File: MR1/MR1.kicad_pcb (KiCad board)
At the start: 2 copper layers, 94 x 71.1 mm, 16 parts, among them J1 Conn_01x04_Male, J2 Conn_01x04_Male, J3 Conn_01x04_Male, J4 Conn_01x04_Male, J5 Conn_01x02_Male, J6 Conn_01x04_Male, J7 Conn_01x04_Male, J8 Conn_01x04_Male, Q1 2SC1815, U5 LPC1768, U6 MPU6050, U7 R3008SB, U8 MCP2561-E-P

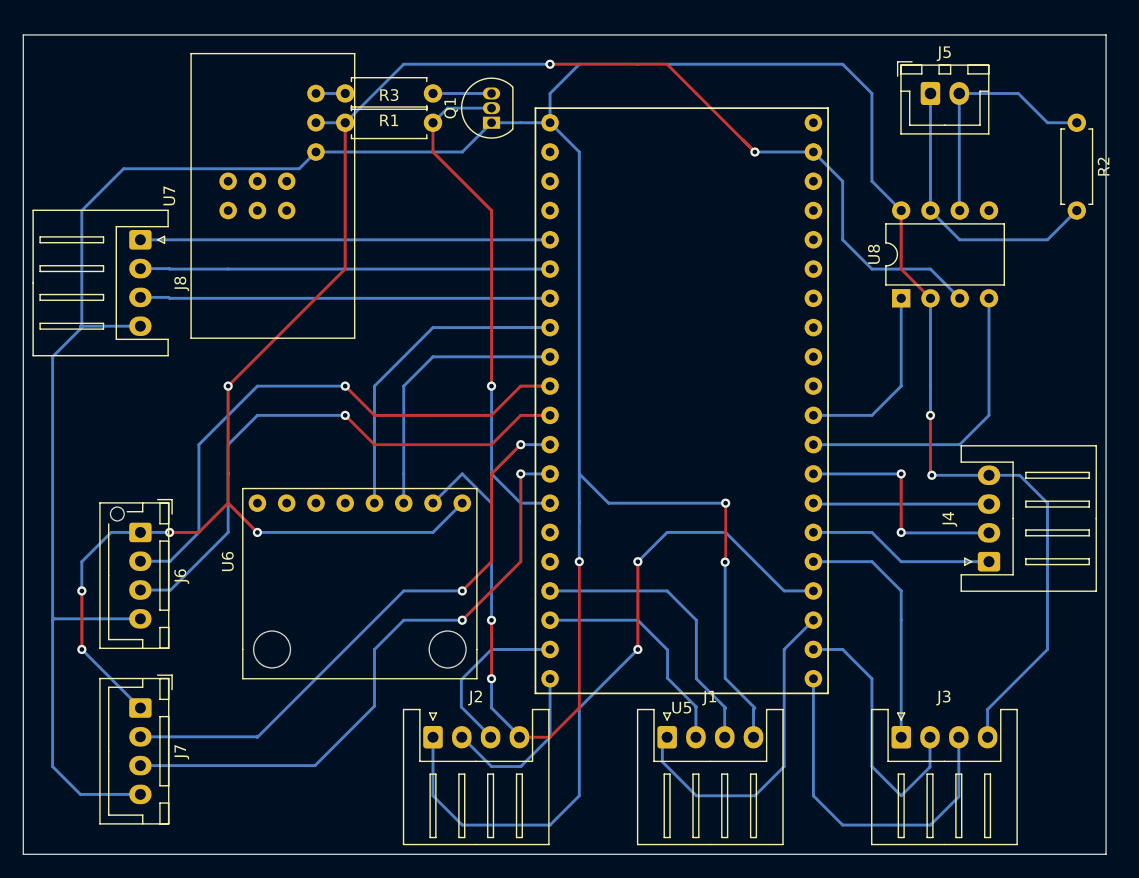
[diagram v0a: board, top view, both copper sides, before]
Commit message: fix: MR1
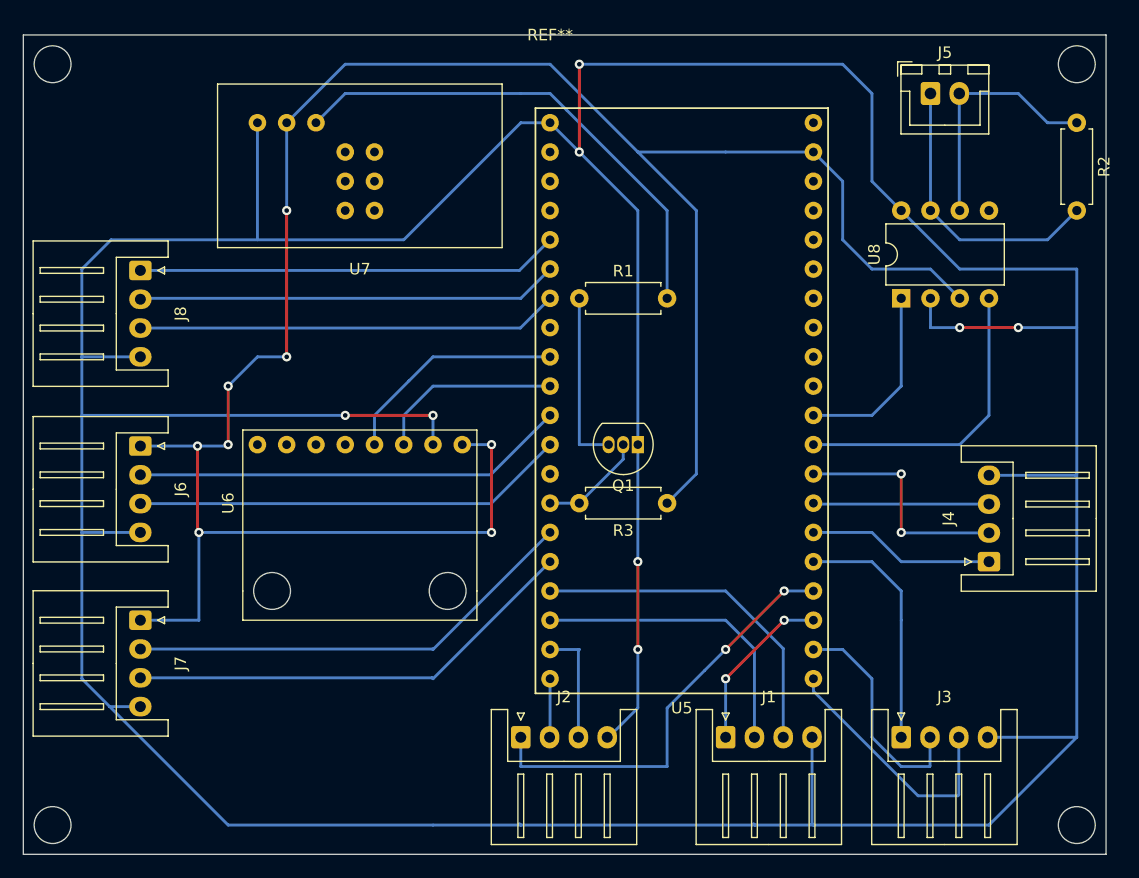
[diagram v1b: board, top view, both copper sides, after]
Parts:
- added REF**: universal_B, MyFootprint:universal_B, F.Cu at (142.2, 99.1)
- J6: footprint Connector_JST:JST_XH_B4B-XH-AM_1x04_P2.50mm_Vertical -> Connector_JST:JST_XH_S4B-XH-A_1x04_P2.50mm_Horizontal
- J7: footprint Connector_JST:JST_XH_B4B-XH-A_1x04_P2.50mm_Vertical -> Connector_JST:JST_XH_S4B-XH-A_1x04_P2.50mm_Horizontal
- moved R3 43.3 mm to (152.4, 104.1), turned to 180 degrees
- moved Q1 30.7 mm to (149.9, 99.1), turned to 180 degrees
- moved R1 21.8 mm to (144.8, 86.4), turned to 0 degrees
- moved J7 7.62 mm to (106.7, 114.3)
- moved J2 7.62 mm to (139.7, 124.5)
- moved J6 7.50 mm to (106.7, 99.2)
- moved U7 7.41 mm to (125.7, 73.7), turned to 0 degrees
- moved U6 5.08 mm to (124.5, 104.1)
- moved J1 5.08 mm to (157.5, 124.5)
- moved J8 2.66 mm to (106.7, 83.9)
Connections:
- U5 pad 10: enc_X_b -> I2C_scl
- U5 pad 11: enc_X_a -> enc_X_b
- U5 pad 12: enc_Y_b -> enc_X_a
- U5 pad 13: enc_Y_a -> Net-(U5-Pad13)
- U5 pad 15: Net-(U5-Pad15) -> enc_Y_b
- U5 pad 16: Net-(U5-Pad16) -> enc_Y_a
- U5 pad 8: I2C_sda -> Net-(U5-Pad8)
- U5 pad 9: I2C_scl -> I2C_sda
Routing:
- net GND: track 337.8 -> 431.8 mm
- net Net-(R1-Pad2): track 2.54 -> 43.4 mm
- net +5V: track 160.2 -> 200.6 mm, vias 7 -> 8
- net Serial_rx: track 44.3 -> 9.20 mm, vias 1 -> 0
- net PWM_2: track 60.7 -> 37.2 mm
- net PWM_1: track 28.7 -> 14.8 mm, vias 0 -> 2
- net enc_Y_a: track 53.4 -> 39.8 mm, vias 2 -> 0
- net I2C_sda: track 32.6 -> 19.9 mm
- net enc_Y_b: track 50.6 -> 39.8 mm, vias 2 -> 0
- net enc_X_a: track 48.4 -> 37.7 mm, vias 2 -> 0
- net enc_X_b: track 48.4 -> 37.7 mm, vias 2 -> 0
- net Net-(Q1-Pad3): track 5.08 -> 15.2 mm
- net IO_2B: track 14.7 -> 5.10 mm
- net I2C_scl: track 23.9 -> 16.3 mm
- net IO_3A: track 30.0 -> 22.5 mm
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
